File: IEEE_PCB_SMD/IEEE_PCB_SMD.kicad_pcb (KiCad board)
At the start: 2 copper layers, 98.9 x 105.4 mm, 23 parts, among them U1 555, U2 4017, U3 EG1218, U4 EG1218, U5 CR2025TR

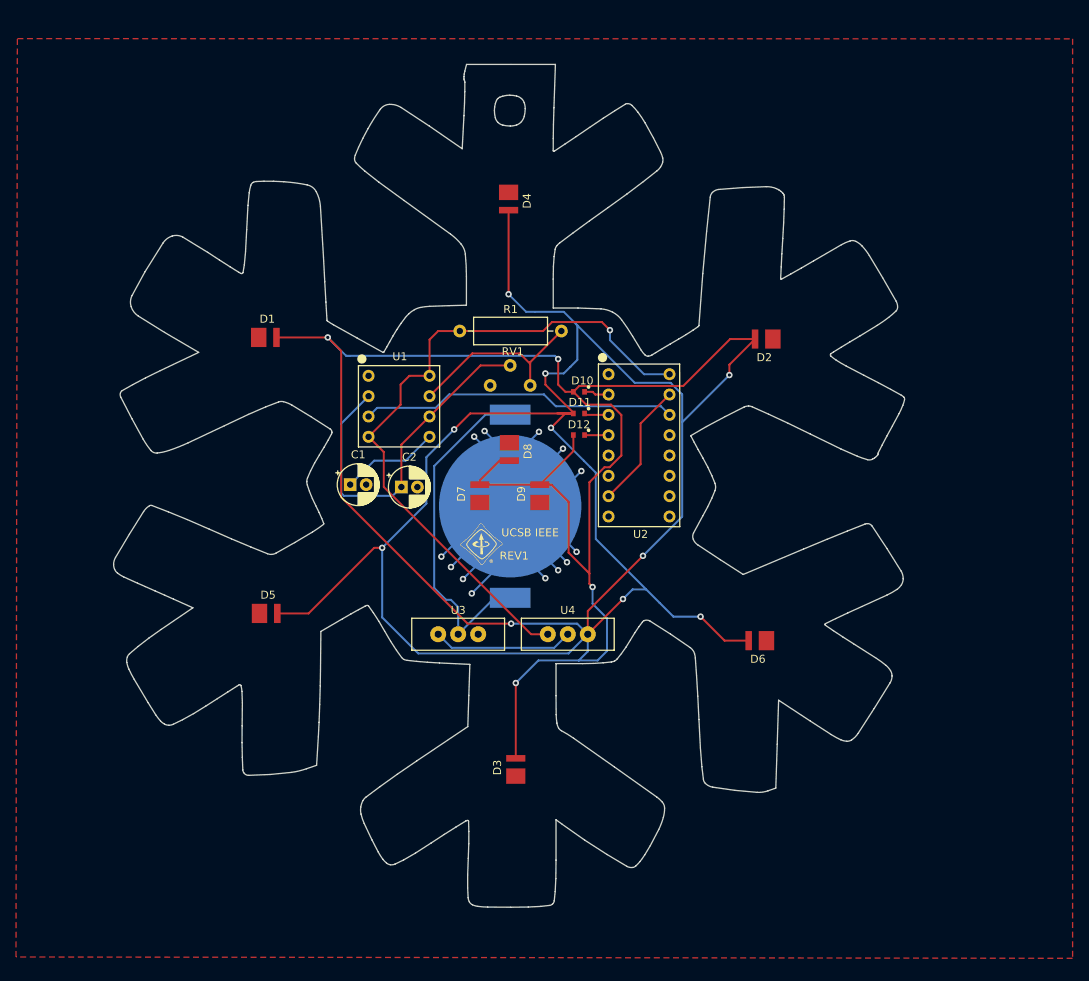
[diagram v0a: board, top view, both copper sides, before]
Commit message: Rev4
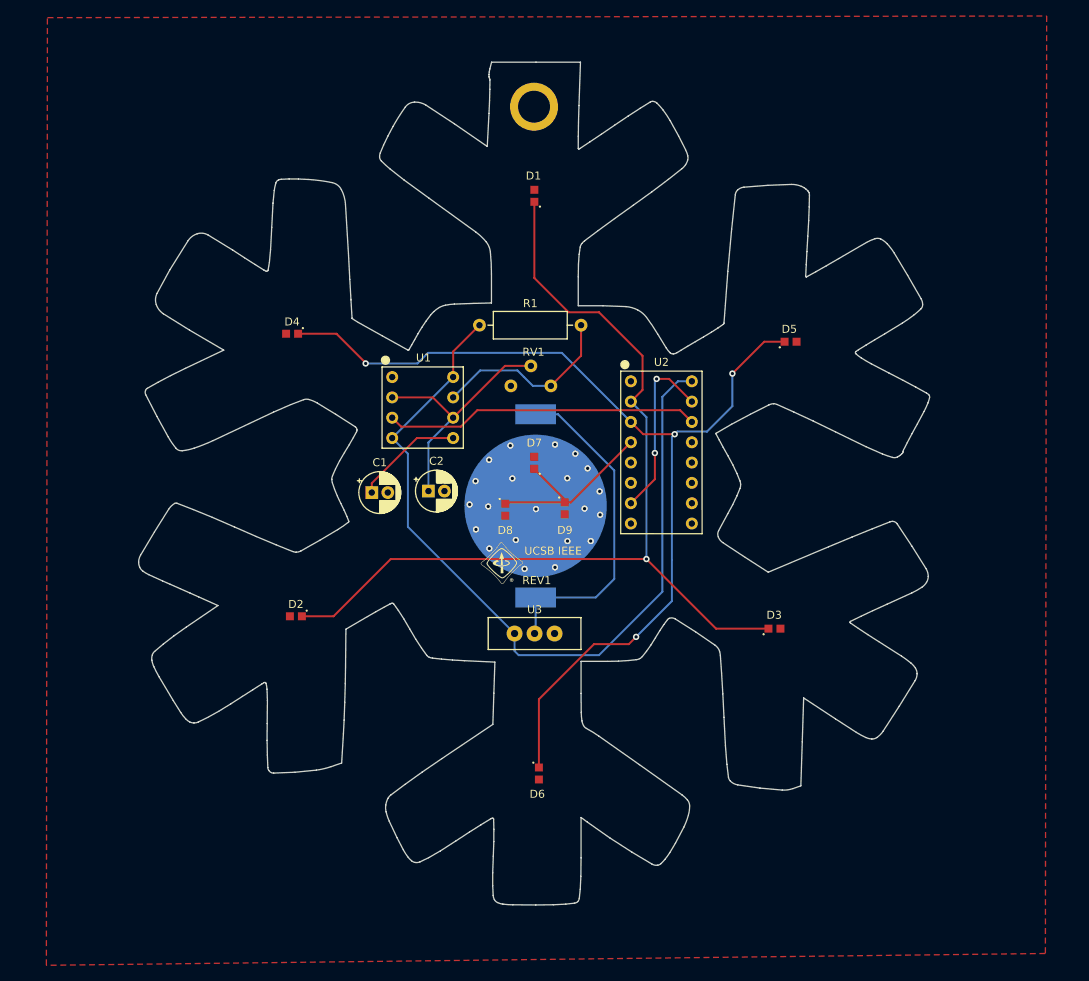
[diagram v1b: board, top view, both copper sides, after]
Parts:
- removed D10, D11, D12: D, IEEE_PCB_Ornament:SDM20U40Q
- removed the G*** at (141.4, 100.6)
- removed U4: EG1218, IEEE_PCB_Ornament:EG1218
- added G***: LOGO, custom parts:IEEE Logo, F.Cu at (143.9, 103.0)
- D1, D2, D3, D4, D5, D6, D7, D8, D9: footprint IEEE_PCB_Ornament:LED_SMD -> IEEE_Ornament:IN-S63AT
- RV1: value 100K -> 50K; footprint IEEE_PCB_Ornament:CT6EP504 -> IEEE_Ornament:CT6EP504
- U1: footprint IEEE_PCB_Ornament:555 -> IEEE_Ornament:555
- U2: footprint IEEE_PCB_Ornament:4017 -> IEEE_Ornament:4017
- U3: footprint IEEE_PCB_Ornament:EG1218 -> IEEE_Ornament:EG1218
- U5: footprint IEEE_PCB_Ornament:CR2025TR -> IEEE_Ornament:CR2025TR
- moved D5 73.8 mm to (180.0, 75.2), turned to 180 degrees
- moved D2 68.2 mm to (118.2, 109.6), turned to 0 degrees
- moved D1 38.0 mm to (148.0, 57.0)
- moved D3 36.8 mm to (178.0, 111.1), turned to 180 degrees
- moved D6 32.2 mm to (148.6, 129.2)
- moved D4 31.9 mm to (117.7, 74.2), turned to 0 degrees
- moved U3 9.55 mm to (148.1, 111.7)
- moved D7 7.95 mm to (148.0, 90.4), turned to -90 degrees
- moved D8 7.55 mm to (144.4, 96.2), turned to 90 degrees
- moved D9 3.50 mm to (151.8, 96.1), turned to 90 degrees
- moved C2 3.42 mm to (134.8, 93.9)
- moved U5 3.18 mm to (148.2, 95.8)
- moved REF** 3.14 mm to (100.5, 99.0)
- moved U1 2.96 mm to (130.3, 79.7)
- moved U2 2.93 mm to (160.1, 80.2)
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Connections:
- D1 pad 2: ALLON -> Net-(D1-Pad2)
- D2 pad 2: ALLON -> Net-(D1-Pad2)
- D3 pad 2: ALLON -> Net-(D1-Pad2)
- D4 pad 2: ALLON -> Net-(D4-Pad2)
- D5 pad 2: ALLON -> Net-(D4-Pad2)
- D6 pad 2: ALLON -> Net-(D4-Pad2)
- D7 pad 2: ALLON -> Net-(D7-Pad2)
- D8 pad 2: ALLON -> Net-(D7-Pad2)
- D9 pad 2: ALLON -> Net-(D7-Pad2)
- U2 pad 1: Net-(U2-Pad1) -> unconnected-(U2-Pad1)
- U2 pad 10: Net-(U2-Pad10) -> unconnected-(U2-Pad10)
- U2 pad 11: Net-(U2-Pad11) -> unconnected-(U2-Pad11)
- U2 pad 12: Net-(U2-Pad12) -> unconnected-(U2-Pad12)
- U2 pad 2: Net-(D10-Pad2) -> Net-(D1-Pad2)
- U2 pad 3: Net-(D11-Pad2) -> Net-(D4-Pad2)
- U2 pad 4: Net-(D12-Pad2) -> Net-(D7-Pad2)
- U2 pad 5: Net-(U2-Pad5) -> unconnected-(U2-Pad5)
- U2 pad 6: Net-(U2-Pad6) -> unconnected-(U2-Pad6)
- U2 pad 9: Net-(U2-Pad9) -> unconnected-(U2-Pad9)
- U3 pad 1: Net-(U3-Pad1) -> +3V3
- U3 pad 3: Net-(U3-Pad3) -> unconnected-(U3-Pad3)
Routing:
- net ALLON: track 472.8 -> 0.00 mm, vias 14 -> 0
- net GND: track 157.5 -> 0.00 mm, vias 13 -> 21
- net Net-(D4-Pad2): track 0.00 -> 125.6 mm, vias 0 -> 4
- net Net-(D1-Pad2): track 0.00 -> 118.8 mm, vias 0 -> 1
- net Net-(D7-Pad2): track 0.00 -> 24.7 mm
- net Net-(U3-Pad1): track 17.6 -> 0.00 mm
- net +3V3: track 86.3 -> 102.4 mm, vias 1 -> 0
- net Net-(C2-Pad1): track 44.7 -> 31.5 mm
- net Net-(U2-Pad15): track 15.9 -> 22.4 mm, vias 0 -> 2
- net Net-(D10-Pad2): track 3.14 -> 0.00 mm
- net Net-(D11-Pad2): track 3.07 -> 0.00 mm
- net Net-(D12-Pad2): track 3.01 -> 0.00 mm
- net Net-(U3-Pad2): track 43.2 -> 41.7 mm
- net Net-(C1-Pad1): track 12.4 -> 13.7 mm
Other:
- board size 98.9 x 105.4 mm -> 98.9 x 105.3 mm
- net class Default removed
